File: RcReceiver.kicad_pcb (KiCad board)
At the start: 2 copper layers, 60 parts, among them J1 VBAT, J13 CAN, J2 SWD, J3 I2C, J4 USART1, J5 Analog input, J6 GPS, J7 SPI3, U1 LP38693-3.3, U2 STM32L476VGT6, U3 LP38693-5.0, U4 TXB0108DQSR, U5 MCP2551, U6 LP38693SD-3.3, Y1 16MHz

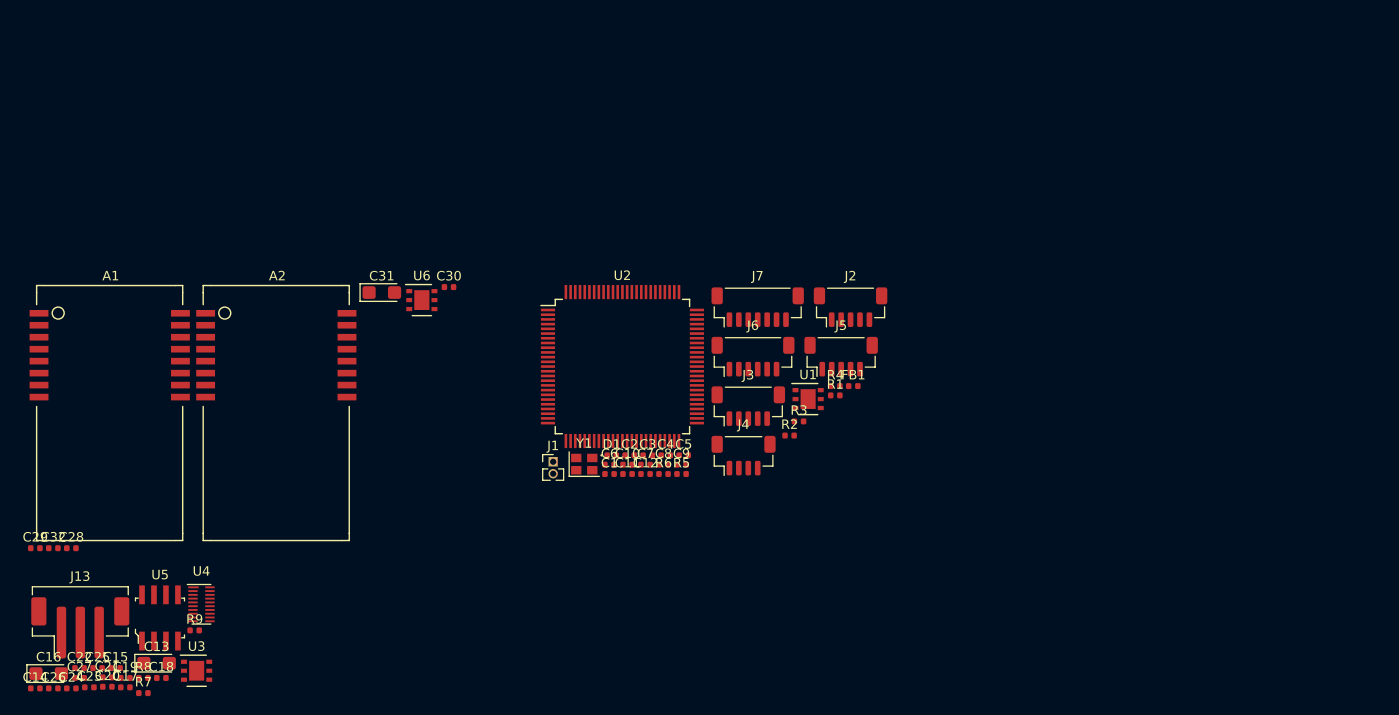
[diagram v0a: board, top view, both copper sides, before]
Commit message: Create PCB
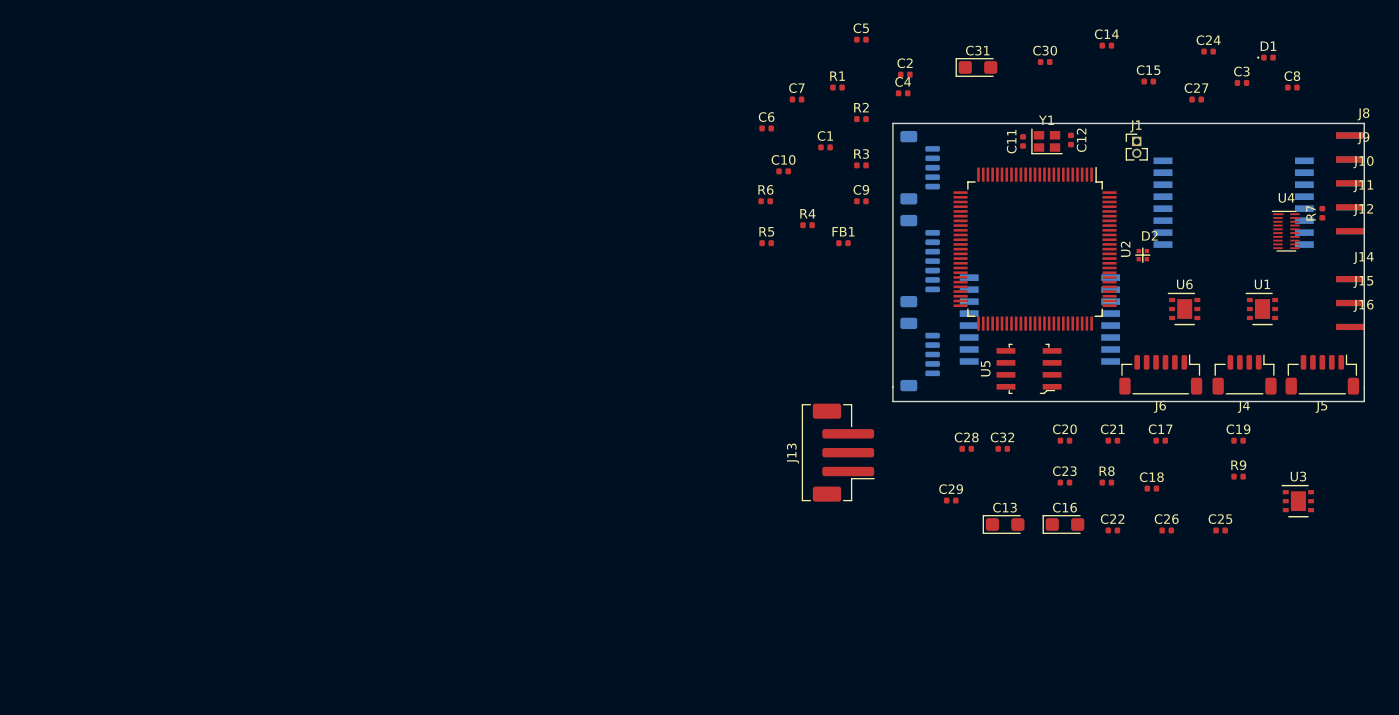
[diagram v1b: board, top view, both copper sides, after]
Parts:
- added D2: LED_ARGB, miscellaneous:LED_Lumex-LX0404, F.Cu at (162.5, 60.0)
- added J10: Servo3, miscellaneous:PinHeader_1x03_P1.27mm_Side, F.Cu at (186.0, 52.4)
- added J11: Servo4, miscellaneous:PinHeader_1x03_P1.27mm_Side, F.Cu at (186.0, 54.9)
- added J12: Servo5, miscellaneous:PinHeader_1x03_P1.27mm_Side, F.Cu at (186.0, 57.4)
- added J14: Servo6, miscellaneous:PinHeader_1x03_P1.27mm_Side, F.Cu at (186.0, 62.5)
- added J15: Servo7, miscellaneous:PinHeader_1x03_P1.27mm_Side, F.Cu at (186.0, 65.0)
- added J16: Servo8, miscellaneous:PinHeader_1x03_P1.27mm_Side, F.Cu at (186.0, 67.6)
- added J8: Servo1, miscellaneous:PinHeader_1x03_P1.27mm_Side, F.Cu at (186.0, 47.3)
- added J9: Servo2, miscellaneous:PinHeader_1x03_P1.27mm_Side, F.Cu at (186.0, 49.8)
- A1, A2, J2, J3, J7: moved to B.Cu
- R5, R6: value 1k -> 470
- moved C24 138.3 mm to (169.5, 38.4)
- moved R7 135.0 mm to (181.6, 55.5), turned to 90 degrees
- moved C27 133.5 mm to (168.2, 43.5)
- moved C14 132.6 mm to (158.7, 37.7)
- moved C15 126.0 mm to (163.1, 41.6)
- moved U4 121.7 mm to (177.7, 57.4)
- moved C19 120.7 mm to (172.7, 79.7)
- moved A1 120.1 mm to (172.0, 60.6), turned to 180 degrees
- moved C25 120.0 mm to (170.8, 89.2)
- moved C26 119.3 mm to (165.0, 89.2)
- moved U3 118.3 mm to (179.0, 86.1)
- moved C17 112.9 mm to (164.4, 79.7)
- moved R9 111.9 mm to (172.7, 83.5)
- moved C22 110.6 mm to (159.3, 89.2)
- moved C21 109.6 mm to (159.3, 79.7)
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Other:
- board outline added: 50 x 29.5 mm
